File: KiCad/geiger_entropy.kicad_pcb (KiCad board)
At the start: 2 copper layers, 114.5 x 130.5 mm, 38 parts, among them J1 AudioJack2, J2 Conn_01x04_Socket, J3 Conn_01x10_Pin, J4 Conn_01x10_Pin, J5 Jack-DC, J6 ICSP, SW1 REV, SW2 FWD, SW3 RESET, U1 LM393, U2 ATmega328-P, U3 L7805, Y1 16MHz

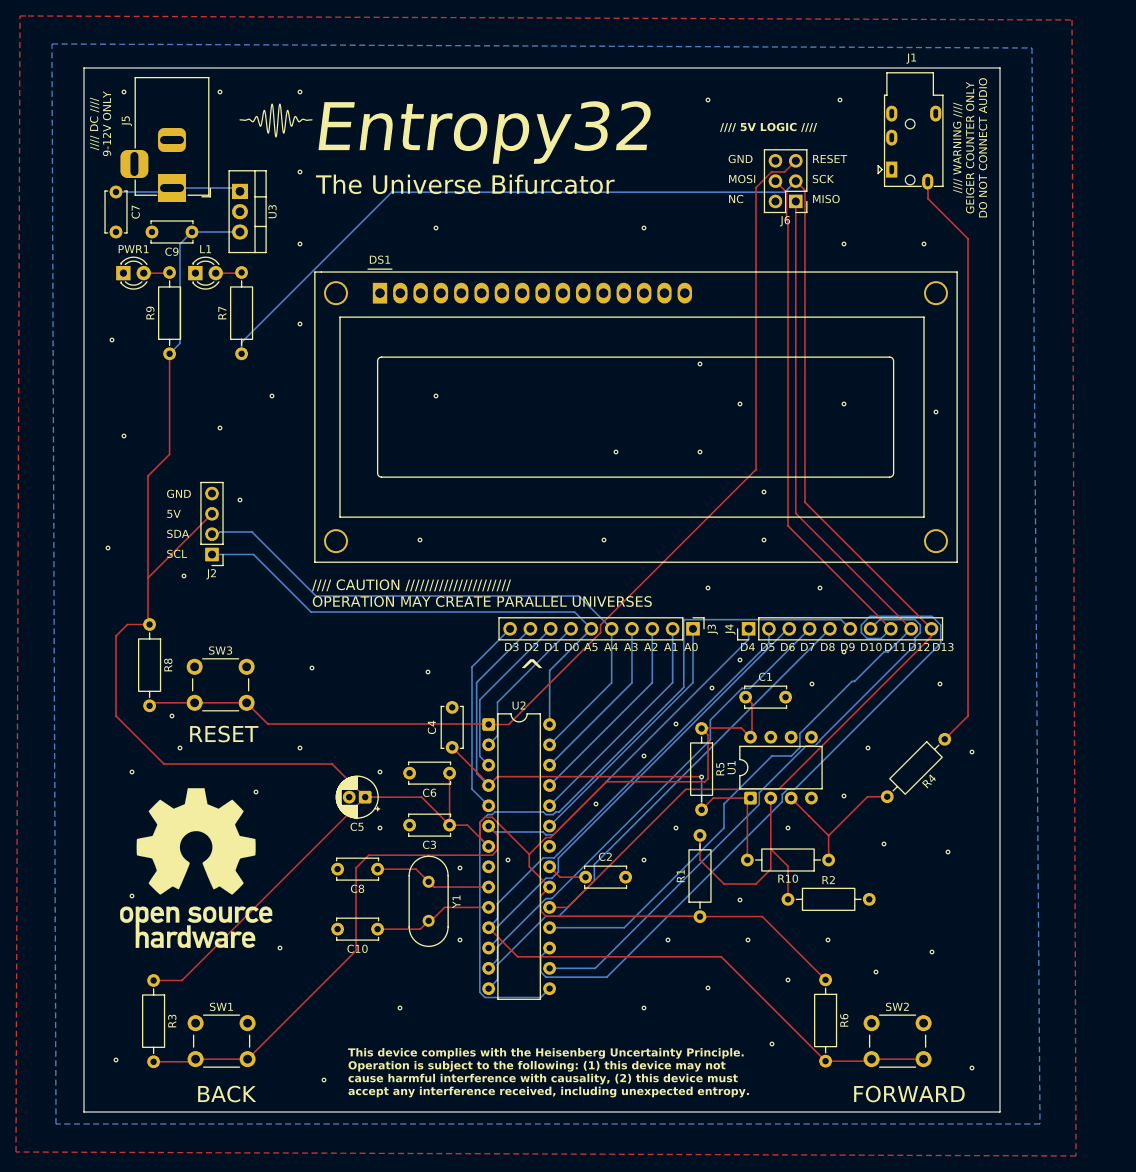
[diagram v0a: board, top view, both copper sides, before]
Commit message: Modify PCB
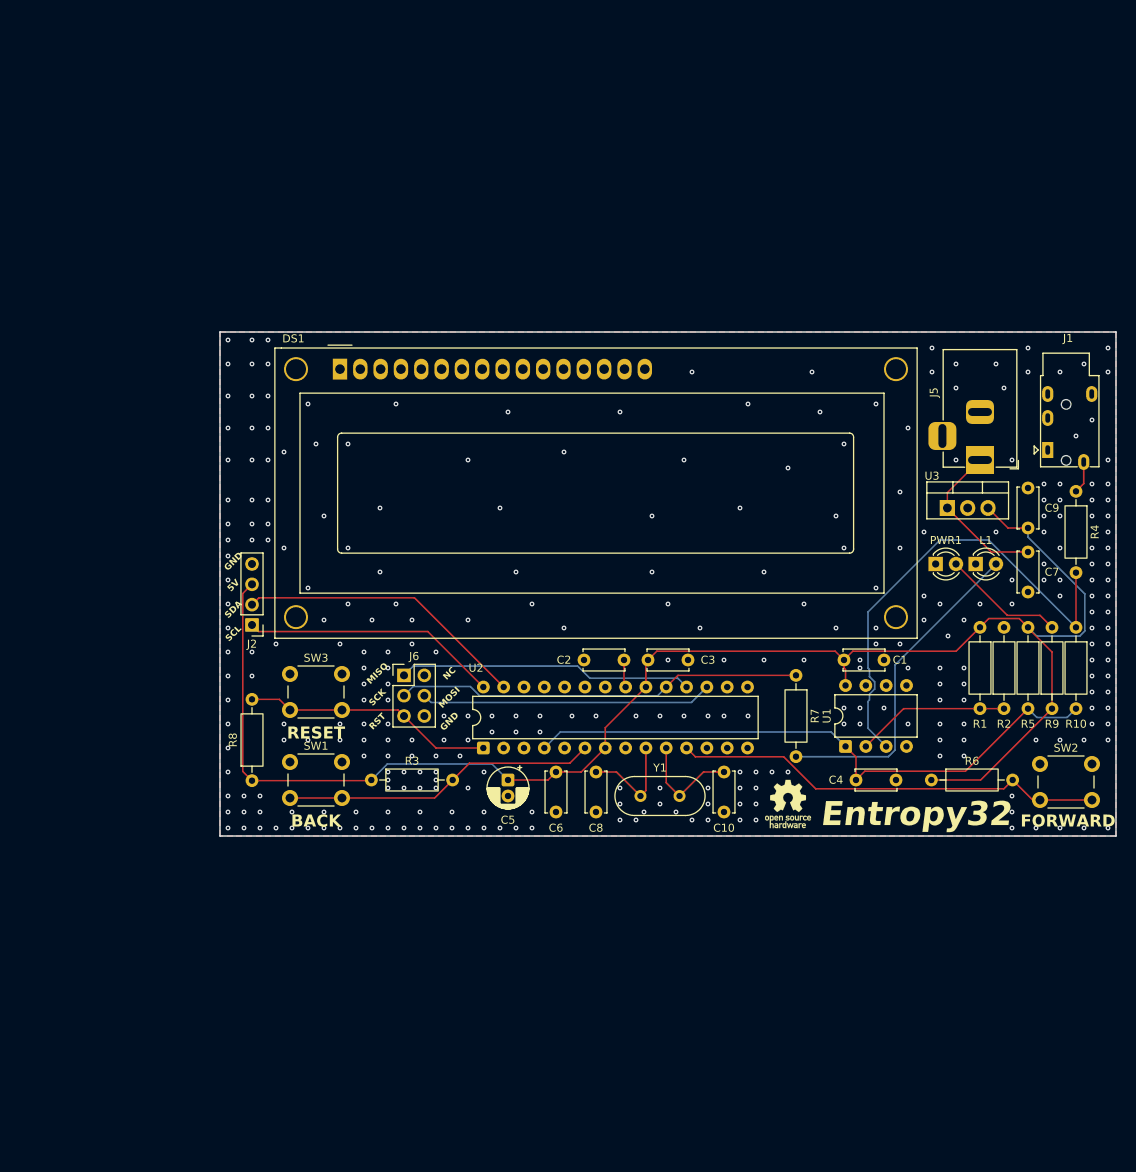
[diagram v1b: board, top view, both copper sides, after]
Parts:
- removed ?: LOGO, Entropy32:wave_packet_logo
- removed J3, J4: Conn_01x10_Pin, Connector_PinHeader_2.54mm:PinHeader_1x10_P2.54mm_Vertical
- removed the REF** at (47.0, 128.0)
- added REF**: OSHW-Logo_5.7x6mm_SilkScreen, Symbol:OSHW-Logo_5.7x6mm_SilkScreen, F.Cu at (121.0, 120.0)
- added REF**: KiCad-Logo2_30mm_SilkScreen, Symbol:KiCad-Logo2_30mm_SilkScreen, B.Cu at (95.0, 79.0)
- moved C7 122.6 mm to (151.0, 88.5)
- moved R9 118.9 mm to (154.0, 108.1)
- moved C9 110.9 mm to (151.0, 85.5), turned to 90 degrees
- moved PWR1 107.8 mm to (139.5, 90.0)
- moved J5 106.6 mm to (145.0, 77.0)
- moved L1 104.1 mm to (144.5, 90.0)
- moved U3 96.9 mm to (140.9, 83.0), turned to 0 degrees
- moved R7 80.1 mm to (122.0, 103.9), turned to -90 degrees
- moved J6 76.9 mm to (73.0, 103.9), turned to 0 degrees
- moved C4 50.6 mm to (129.5, 117.0), turned to 0 degrees
- moved R1 50.3 mm to (145.0, 97.9), turned to -90 degrees
- moved C10 47.5 mm to (113.0, 116.0), turned to -90 degrees
- moved R5 42.7 mm to (151.0, 97.9)
- moved R10 42.4 mm to (157.0, 97.9), turned to -90 degrees
- moved J1 40.1 mm to (153.5, 75.8)
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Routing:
- net /D13/SCK: track 204.8 -> 51.0 mm
- net /D11/MOSI: track 152.0 -> 36.5 mm
- net /RESET: track 133.1 -> 31.4 mm
- net /D9: track 93.2 -> 0.00 mm
- net /D12/MISO: track 122.9 -> 36.9 mm
- net +5V: track 283.8 -> 200.3 mm
- net /D10: track 73.1 -> 0.00 mm
- net Net-(J1-PadS): track 73.0 -> 4.07 mm
- net /D4: track 107.9 -> 39.5 mm
- net /D8: track 63.6 -> 0.00 mm
- net /D7: track 60.1 -> 0.00 mm
- net /D5: track 114.0 -> 54.3 mm
- net /D6: track 56.0 -> 0.00 mm
- net /Geiger_pulse: track 19.0 -> 59.5 mm
- net Net-(L1-A): track 3.26 -> 41.2 mm
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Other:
- board size 114.5 x 130.5 mm -> 112 x 63 mm
- board text added: "RST"
- board text removed: "//// 5V LOGIC ////"
- board text removed: "//// CAUTION ////////////////////// OPERATION MAY CREATE PARALLEL UNIVERSES"
- board text removed: "//// DC //// 9-12V ONLY"
- board text removed: "//// WARNING //// GEIGER COUNTER ONLY DO NOT CONNECT AUDIO"
- board text removed: "A0"
- board text removed: "A1"
- board text removed: "A2"
- board text removed: "A3"
- board text removed: "A4"
- board text removed: "A5"
- board text removed: "D0"
- board text removed: "D1"
- board text removed: "D10"
- board text removed: "D11"
- board text removed: "D12"
- board text removed: "D13"
- board text removed: "D2"
- board text removed: "D3"
- board text removed: "D4"
- board text removed: "D5"
- board text removed: "D6"
- board text removed: "D7"
- board text removed: "D8"
- board text removed: "D9"
- board text removed: "The Universe Bifurcator"
- board text removed: "This device complies with the Heisenberg Uncertainty Principle. Operation is subject to the following: (1) this device may not cause harmful interference with causality, (2) this device must accept any interference received, including unexpected entropy."
- board text removed: "^"
